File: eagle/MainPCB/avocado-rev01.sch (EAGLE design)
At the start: 10 parts, among them J1 10118194-0001LF, J2 CON-DSUB-15-VGA, J3 0475710001, U1 V3S

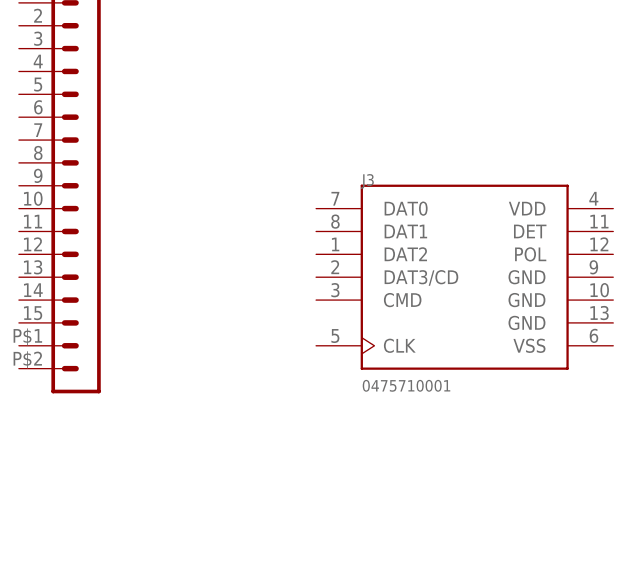
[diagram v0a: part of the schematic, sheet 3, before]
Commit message: updated schematic
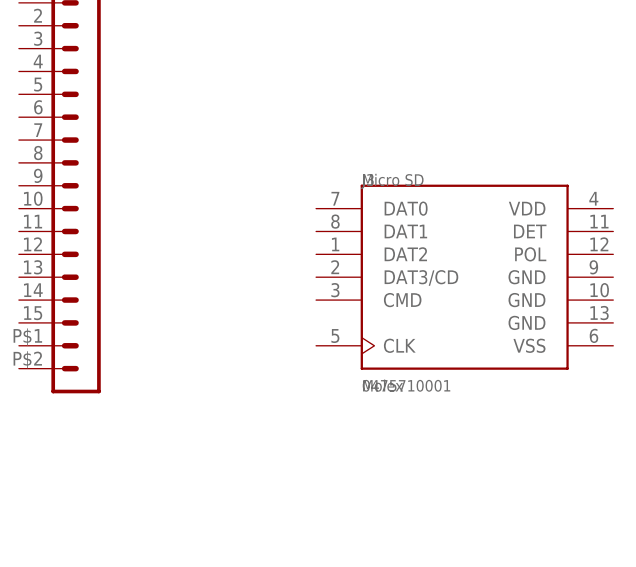
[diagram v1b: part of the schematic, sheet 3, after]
